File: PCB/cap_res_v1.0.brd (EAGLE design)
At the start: 60 x 60 mm, 0 parts

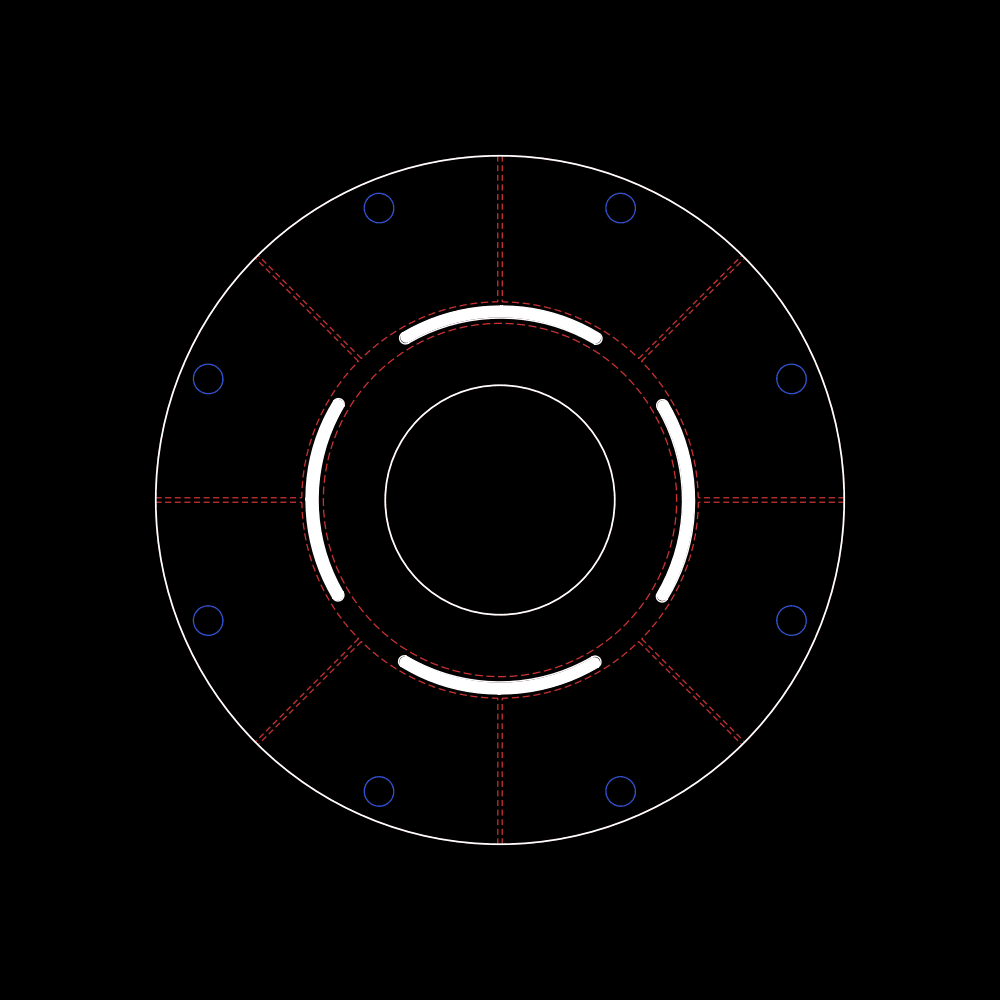
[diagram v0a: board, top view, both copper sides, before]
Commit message: final_version of v1.0 HW
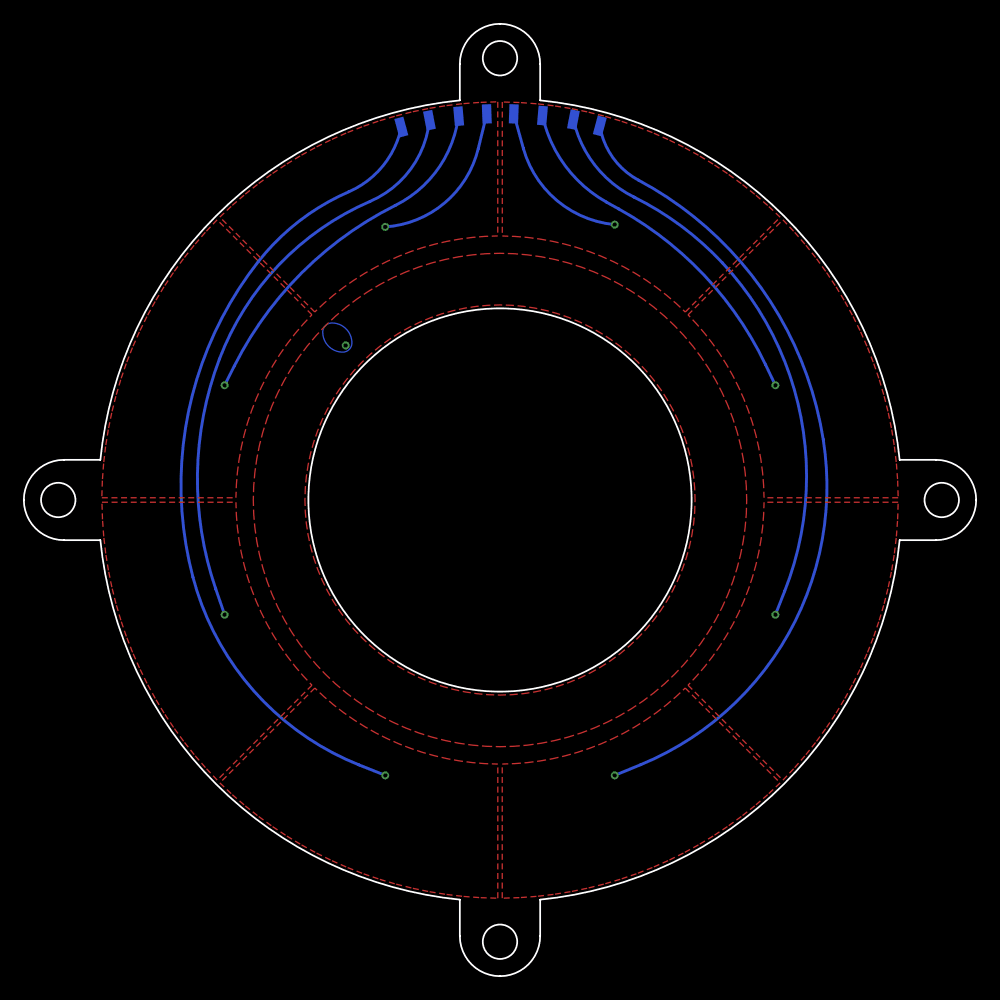
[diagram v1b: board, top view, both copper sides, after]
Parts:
- added U$1: CAPRES_PADS, connectors:CAPRES_PADS
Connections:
- new net S00: U$1.P7
- new net S01: U$1.P6
- new net S02: U$1.P5
- new net S03: U$1.P4
- new net S04: U$1.P3
- new net S05: U$1.P2
- new net S06: U$1.P1
- new net S07: U$1.P0
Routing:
- net S04: track 0.00 -> 69.6 mm, vias 0 -> 1
- net S03: track 0.00 -> 68.5 mm, vias 0 -> 1
- net S05: track 0.00 -> 50.2 mm, vias 0 -> 1
- net S02: track 0.00 -> 49.5 mm, vias 0 -> 1
- net S06: track 0.00 -> 32.3 mm, vias 0 -> 1
- net S01: track 0.00 -> 31.2 mm, vias 0 -> 1
- net S07: track 0.00 -> 13.7 mm, vias 0 -> 1
- net S00: track 0.00 -> 13.5 mm, vias 0 -> 1
- net RX: track 0.00 -> 0.02 mm, vias 0 -> 1
- added copper zone on layer 16, net RX
- removed copper zone on layer 16, net S
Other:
- board size 60 x 60 mm -> 83 x 83 mm
